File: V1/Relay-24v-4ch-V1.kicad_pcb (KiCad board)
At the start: 2 copper layers, 53 x 67.8 mm, 25 parts, among them J1 Conn_01x05, J2 OUT1, J3 OUT2, J4 OUT3, J5 OUT4, K1 G5PZ-1A, K2 G5PZ-1A, K3 G5PZ-1A, K4 G5PZ-1A

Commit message: Adjustments for fabrication
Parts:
- D3, D4, D7, D8: value BLUE/0603 -> GREEN/0603
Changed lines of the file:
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@@
     (property "Case" "0603")
     (property "JLCPCB BOM" "1")
-    (property "LCSC Part #" "C72041")
+    (property "LCSC Part #" "C72043")
     (property "Mfr" "Everlight")
-    (property "Mfr PN" "19-217/BHC-ZL1M2RY/3T")
+    (property "Mfr PN" "19-217/GHC-YR1S2/3T")
     (property "Sheetfile" "Relay-24v-4ch-V1.kicad_sch")
     (property "Sheetname" "")
     (property "Technology" "")
     (property "Vendor" "JLCPCB")
-    (property "Vendor PN" "C72041")
+    (property "Vendor PN" "C72043")
     (property "ki_description" "Light emitting diode")
     (property "ki_keywords" "LED diode")
@@
         (effects (font (size 1 1) (thickness 0.15)))
     )
-    (fp_text value "BLUE/0603" (at 0 1.43) (layer "F.Fab")
+    (fp_text value "GREEN/0603" (at 0 1.43) (layer "F.Fab")
         (effects (font (size 1 1) (thickness 0.15)))
     )
@@
     (property "Case" "0603")
     (property "JLCPCB BOM" "1")
-    (property "LCSC Part #" "C72041")
+    (property "LCSC Part #" "C72043")
     (property "Mfr" "Everlight")
-    (property "Mfr PN" "19-217/BHC-ZL1M2RY/3T")
+    (property "Mfr PN" "19-217/GHC-YR1S2/3T")
     (property "Sheetfile" "Relay-24v-4ch-V1.kicad_sch")
     (property "Sheetname" "")
     (property "Technology" "")
     (property "Vendor" "JLCPCB")
-    (property "Vendor PN" "C72041")
+    (property "Vendor PN" "C72043")
     (property "ki_description" "Light emitting diode")
     (property "ki_keywords" "LED diode")
@@
         (effects (font (size 1 1) (thickness 0.15)))
     )
-    (fp_text value "BLUE/0603" (at 0 1.43) (layer "F.Fab")
+    (fp_text value "GREEN/0603" (at 0 1.43) (layer "F.Fab")
         (effects (font (size 1 1) (thickness 0.15)))
     )
@@
   (footprint "Tales:TerminalBlock_DG141V-2.54-5P_1x05_P2.54mm_Vertical" (layer "F.Cu")
     (at 140.97 62.865 180)
-    (property "Sheetfile" "Relay-24v-4ch-V1.kicad_sch")
-    (property "Sheetname" "")
+    (property "Case" "")
+    (property "JLCPCB BOM" "1")
+    (property "LCSC Part #" "C2898747")
+    (property "Mfr" "Dibo")
+    (property "Mfr PN" "DB141V-2.54-5P")
+    (property "Sheetfile" "Relay-24v-4ch-V1.kicad_sch")
+    (property "Sheetname" "")
+    (property "Technology" "")
+    (property "Vendor" "JLCPCB")
+    (property "Vendor PN" "C2898747")
     (property "ki_description" "Generic connector, single row, 01x05, script generated (kicad-library-utils/schlib/autogen/connector/)")
     (property "ki_keywords" "connector")
@@
     (property "Case" "0603")
     (property "JLCPCB BOM" "1")
-    (property "LCSC Part #" "C72041")
+    (property "LCSC Part #" "C72043")
     (property "Mfr" "Everlight")
-    (property "Mfr PN" "19-217/BHC-ZL1M2RY/3T")
+    (property "Mfr PN" "19-217/GHC-YR1S2/3T")
     (property "Sheetfile" "Relay-24v-4ch-V1.kicad_sch")
     (property "Sheetname" "")
     (property "Technology" "")
     (property "Vendor" "JLCPCB")
-    (property "Vendor PN" "C72041")
+    (property "Vendor PN" "C72043")
     (property "ki_description" "Light emitting diode")
     (property "ki_keywords" "LED diode")
@@
         (effects (font (size 1 1) (thickness 0.15)))
     )
-    (fp_text value "BLUE/0603" (at 0 1.43) (layer "F.Fab")
+    (fp_text value "GREEN/0603" (at 0 1.43) (layer "F.Fab")
         (effects (font (size 1 1) (thickness 0.15)))
     )
@@
     (property "Case" "0603")
     (property "JLCPCB BOM" "1")
-    (property "LCSC Part #" "C72041")
+    (property "LCSC Part #" "C72043")
     (property "Mfr" "Everlight")
-    (property "Mfr PN" "19-217/BHC-ZL1M2RY/3T")
+    (property "Mfr PN" "19-217/GHC-YR1S2/3T")
     (property "Sheetfile" "Relay-24v-4ch-V1.kicad_sch")
     (property "Sheetname" "")
     (property "Technology" "")
     (property "Vendor" "JLCPCB")
-    (property "Vendor PN" "C72041")
+    (property "Vendor PN" "C72043")
     (property "ki_description" "Light emitting diode")
     (property "ki_keywords" "LED diode")
@@
         (effects (font (size 1 1) (thickness 0.15)))
     )
-    (fp_text value "BLUE/0603" (at 0 1.43) (layer "F.Fab")
-        (effects (font (size 1 1) (thickness 0.15)))
-    )
+    (fp_text value "GREEN/0603" (at 0 1.43) (layer "F.Fab")
+        (effects (font (size 1 1) (thickness 0.15)))
+    )

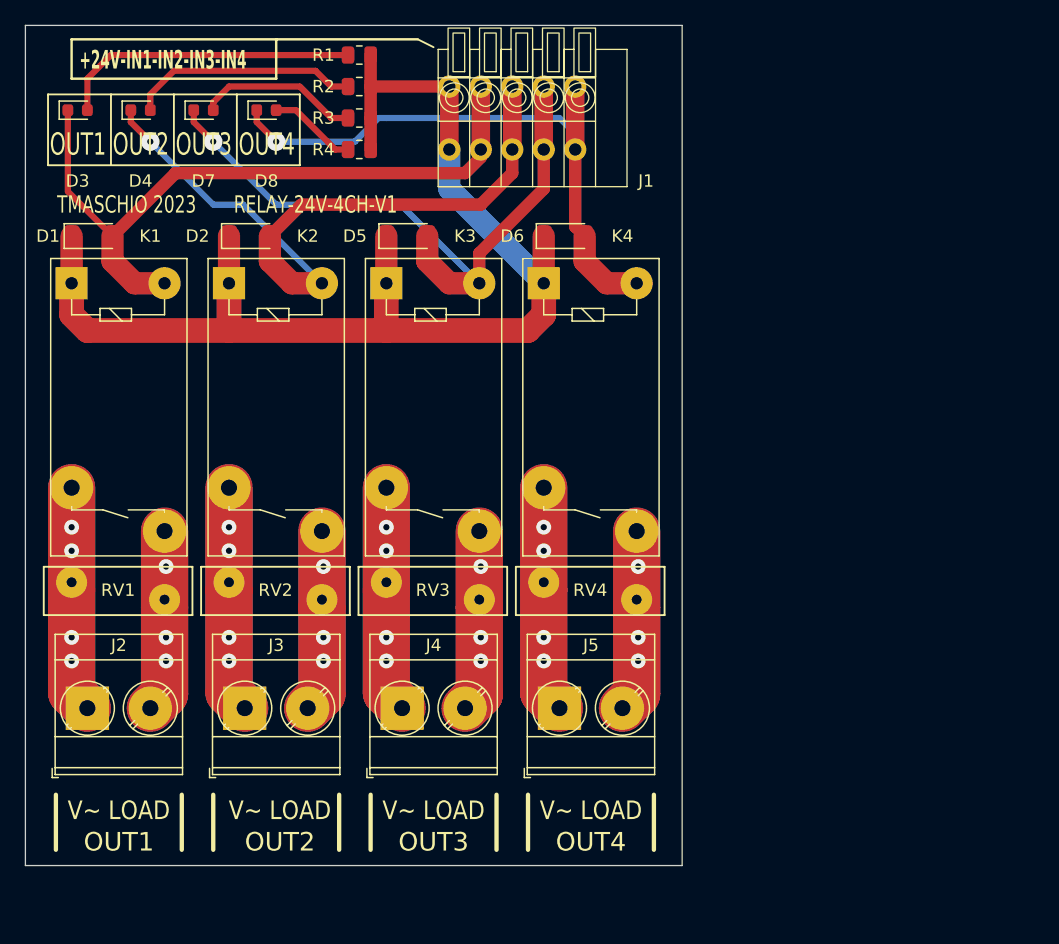
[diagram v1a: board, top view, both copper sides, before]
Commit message: Redone everything
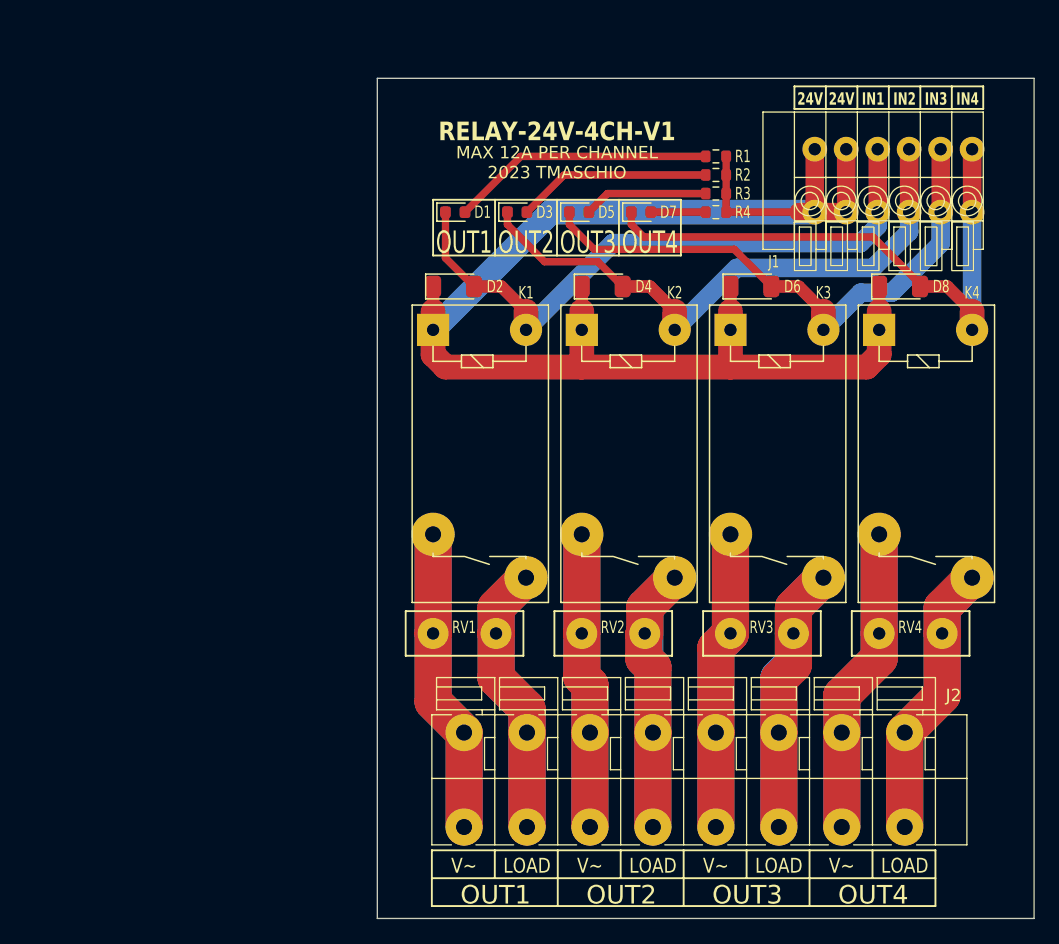
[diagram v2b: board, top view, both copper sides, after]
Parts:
- removed J3: OUT2, Tales:TerminalBlock_Phoenix_MKDS-3-2-5.08_1x02_P5.08mm_Horizontal
- removed J4: OUT3, Tales:TerminalBlock_Phoenix_MKDS-3-2-5.08_1x02_P5.08mm_Horizontal
- removed J5: OUT4, Tales:TerminalBlock_Phoenix_MKDS-3-2-5.08_1x02_P5.08mm_Horizontal
- D1: renamed from D3; value GREEN/0603 -> GREEN
- D2: renamed from D1; value 1N4148/SOD-123 -> 1N4148
- D3: renamed from D4; value GREEN/0603 -> GREEN
- D4: renamed from D2; value 1N4148/SOD-123 -> 1N4148
- D5: renamed from D7; value GREEN/0603 -> GREEN
- D6: renamed from D5; value 1N4148/SOD-123 -> 1N4148
- D7: renamed from D8; value GREEN/0603 -> GREEN
- D8: renamed from D6; value 1N4148/SOD-123 -> 1N4148
- J1: value Conn_01x05 -> DG141V-2.54-6P; footprint Tales:TerminalBlock_DG141V-2.54-5P_1x05_P2.54mm_Vertical -> Tales:TerminalBlock_Dibo_DB141V-2.54-6P_1x06_P2.54mm_Vertical
- J2: value OUT1 -> DB142V-5.08-8P; footprint Tales:TerminalBlock_Phoenix_MKDS-3-2-5.08_1x02_P5.08mm_Horizontal -> Tales:TerminalBlock_Dibo_DB142V-5.08-8P_1x08_P5.08mm_Vertical
- K1, K2, K3, K4: footprint Tales:Relay_SPST_Omron-G5PZ-1A -> Tales:Relay_SPST_Omron_G5PZ-1A
- R1, R2, R3, R4: value 4k7/0,125W/0805 -> 5k6/100mW; footprint Tales:R_0805_2012Metric -> Tales:R_0603_1608Metric
- RV1, RV2, RV3, RV4: value 250VAC -> 275VAC; footprint Tales:RV_Disc_D12mm_W3.9mm_P7.5mm -> Tales:RV_Disc_D9.50mm_W3.6mm_P5.08mm
- moved J1 32.4 mm to (173.0, 67.9)
- moved J2 31.9 mm to (132.0, 122.6)
- moved D1 31.6 mm to (131.3, 73.0)
- moved D3 31.5 mm to (136.3, 73.0)
- moved D5 31.4 mm to (141.3, 73.0)
- moved D7 31.3 mm to (146.3, 73.0)
- moved R1 29.9 mm to (152.3, 68.5)
- moved R2 29.6 mm to (152.3, 70.0)
- moved RV1 29.5 mm to (129.5, 107.0)
- moved D2 29.5 mm to (131.2, 79.0)
- moved R3 29.4 mm to (152.3, 71.5)
- moved K1 29.4 mm to (129.5, 82.5)
- moved R4 29.2 mm to (152.3, 73.0)
- moved RV2 28.8 mm to (141.5, 107.0)
- moved D4 28.8 mm to (143.2, 79.0)
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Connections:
- K2 pad 2: Net-(J3-Pin_1) -> Net-(J2-Pin_3)
- K2 pad 3: Net-(J3-Pin_2) -> Net-(J2-Pin_4)
- K3 pad 2: Net-(J4-Pin_1) -> Net-(J2-Pin_5)
- K3 pad 3: Net-(J4-Pin_2) -> Net-(J2-Pin_6)
- K4 pad 2: Net-(J5-Pin_1) -> Net-(J2-Pin_7)
- K4 pad 3: Net-(J5-Pin_2) -> Net-(J2-Pin_8)
- RV2 pad 1: Net-(J3-Pin_1) -> Net-(J2-Pin_3)
- RV2 pad 2: Net-(J3-Pin_2) -> Net-(J2-Pin_4)
- RV3 pad 1: Net-(J4-Pin_1) -> Net-(J2-Pin_5)
- RV3 pad 2: Net-(J4-Pin_2) -> Net-(J2-Pin_6)
- RV4 pad 1: Net-(J5-Pin_1) -> Net-(J2-Pin_7)
- RV4 pad 2: Net-(J5-Pin_2) -> Net-(J2-Pin_8)
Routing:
- net Net-(J2-Pin_7): track 0.00 -> 49.7 mm
- net Net-(J2-Pin_5): track 0.00 -> 48.2 mm
- net Net-(J2-Pin_3): track 0.00 -> 47.8 mm
- net Net-(J2-Pin_8): track 0.00 -> 44.7 mm
- net Net-(J2-Pin_6): track 0.00 -> 43.2 mm
- net Net-(J2-Pin_4): track 0.00 -> 42.9 mm
- net Net-(J4-Pin_1): track 36.6 -> 0.00 mm, vias 4 -> 0
- net Net-(J3-Pin_1): track 36.6 -> 0.00 mm, vias 4 -> 0
- net Net-(J5-Pin_1): track 36.6 -> 0.00 mm, vias 4 -> 0
- net Net-(J5-Pin_2): track 29.5 -> 0.00 mm, vias 3 -> 0
- net Net-(J3-Pin_2): track 29.5 -> 0.00 mm, vias 3 -> 0
- net Net-(J4-Pin_2): track 29.5 -> 0.00 mm, vias 3 -> 0
- net +24V: track 100.1 -> 119.9 mm
- net Net-(J2-Pin_2): track 29.5 -> 44.3 mm, vias 3 -> 0
- net Net-(J2-Pin_1): track 36.6 -> 49.3 mm, vias 4 -> 0
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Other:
- board text added: "24V"
- board text added: "CORRENTE MÁXIMA POR CANAL CONSIDERAÇÕES: - ESPESSURA COBRE 0,035mm, TRILHAS EM AMBOS LAYERS, EQUIVALE 0,070mm - deltaT NA TRILHA 20ºC - LARGURA DE TRILHA NECESSÁRIA PARA 12A = 3,03726mm TRILHAS DESENHADAS EM AMBOS OS LAYERS COM 3,1mm DE LARGURA"
- board text added: "IN1"
- board text added: "IN2"
- board text added: "IN3"
- board text added: "IN4"
- board text added: "LOAD"
- board text added: "MAX 12A PER CHANNEL 2023 TMASCHIO"
- board text added: "V~"
- board text removed: "+24V-IN1-IN2-IN3-IN4"
- board text removed: "TMASCHIO 2023"
- board text removed: "V~ LOAD"
